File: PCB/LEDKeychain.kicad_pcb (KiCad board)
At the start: 2 copper layers, 32 x 49.5 mm, 37 parts, among them U1 13.56MHz

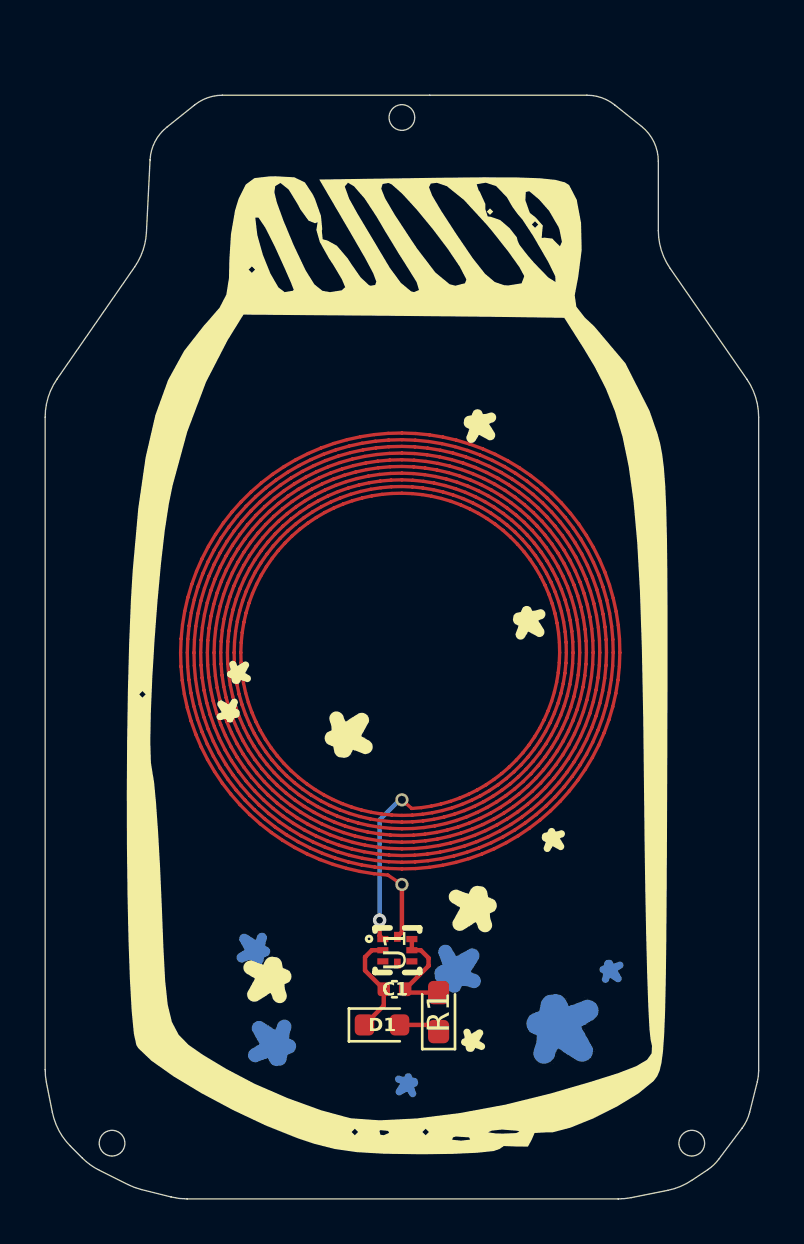
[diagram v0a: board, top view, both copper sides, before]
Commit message: Add files via upload
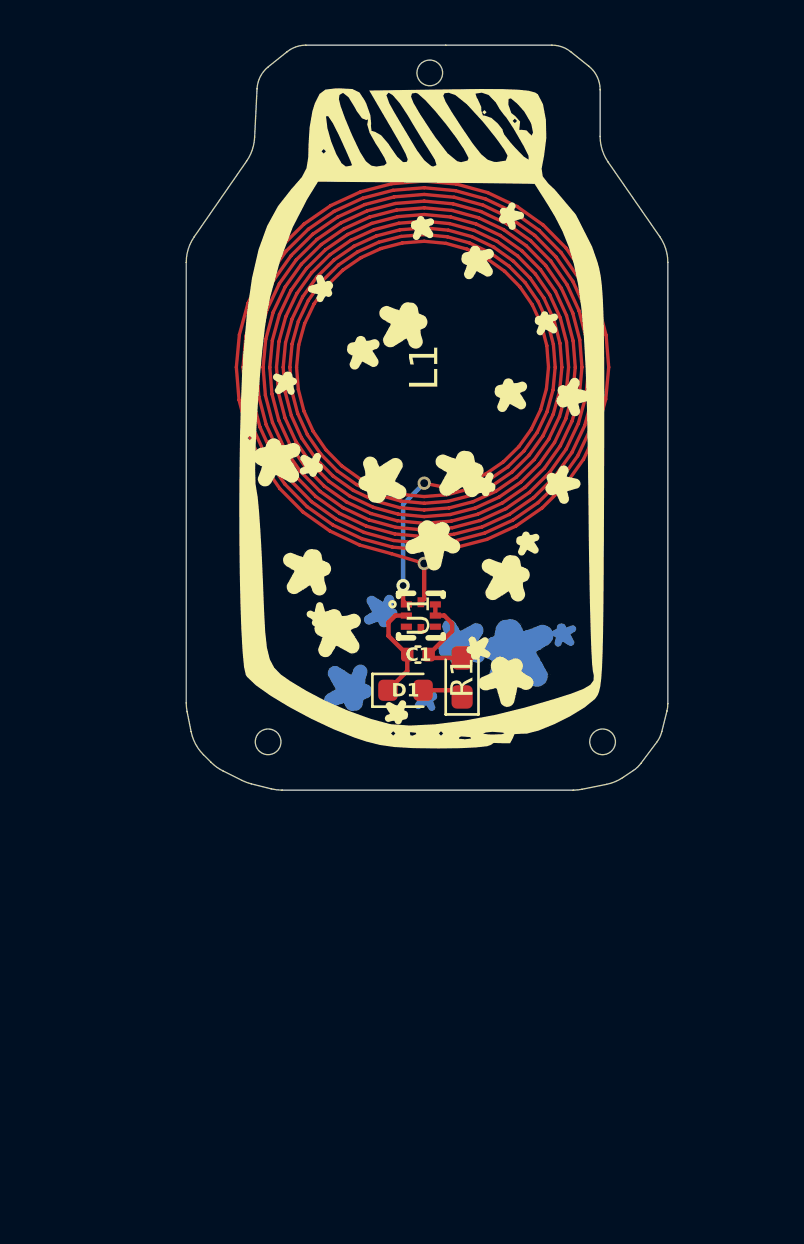
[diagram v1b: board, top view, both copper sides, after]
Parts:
- removed the REF** at (131.0, 93.0)
- removed the REF** at (144.0, 115.0)
- removed the REF** at (118.0, 115.0)
- removed the REF** at (131.0, 69.0)
- added G***: LOGO, LOGO, F.Cu at (137.7, 78.8)
- added G***: LOGO, LOGO, F.Cu at (125.8, 85.7)
- added G***: LOGO, LOGO, F.Cu at (134.5, 84.9)
- added G***: LOGO, LOGO, F.Cu at (130.5, 95.1)
- added G***: LOGO, LOGO, F.Cu at (136.4, 73.7)
- added G***: LOGO, LOGO, F.Cu at (128.5, 93.3)
- added G***: LOGO, LOGO, F.Cu at (129.6, 80.4)
- added G***: LOGO, LOGO, F.Cu at (127.6, 90.8)
- added G***: LOGO, LOGO, F.Cu at (139.5, 81.9)
- added G***: LOGO, LOGO, F.Cu at (129.9, 78.7)
- added G***: LOGO, LOGO, F.Cu at (139.0, 85.8)
- added G***: LOGO, LOGO, B.Cu at (133.7, 88.5)
- added G***: LOGO, LOGO, B.Cu at (135.7, 83.3)
- added G***: LOGO, LOGO, B.Cu at (130.0, 87.9)
- added G***: LOGO, LOGO, B.Cu at (136.8, 88.5)
- added G***: LOGO, LOGO, B.Cu at (128.0, 89.8)
- added G***: LOGO, LOGO, F.Cu at (132.4, 85.4)
- added G***: LOGO, LOGO, B.Cu at (131.9, 74.6)
- added G***: LOGO, LOGO, B.Cu at (126.4, 77.1)
- added G***: LOGO, LOGO, B.Cu at (127.7, 85.9)
- added G***: LOGO, LOGO, B.Cu at (132.3, 79.2)
- added G***: LOGO, LOGO, B.Cu at (138.4, 85.8)
- added G***: LOGO, LOGO, F.Cu at (135.1, 95.4)
- added G***: LOGO, LOGO, B.Cu at (137.2, 86.7)
- added G***: LOGO, LOGO, B.Cu at (136.3, 73.6)
- added G***: LOGO, LOGO, B.Cu at (125.2, 82.0)
- added G***: LOGO, LOGO, F.Cu at (132.1, 74.6)
- added G***: LOGO, LOGO, B.Cu at (135.1, 91.4)
- added G***: LOGO, LOGO, B.Cu at (129.5, 88.9)
- added G***: LOGO, LOGO, F.Cu at (131.8, 89.3)
- added G***: LOGO, LOGO, F.Cu at (125.2, 81.1)
- added G***: LOGO, LOGO, F.Cu at (126.8, 76.4)
- added L1: L, Antenna:Antenna_8500000x5500000mm, F.Cu at (132.0, 80.2)
- added REF**: ToolingHole_1.152mm, MountingHole:ToolingHole_1.152mm, F.Cu at (140.0, 97.0)
- added REF**: ToolingHole_1.152mm, MountingHole:ToolingHole_1.152mm, F.Cu at (125.0, 97.0)
- added REF**: ToolingHole_1.152mm, MountingHole:ToolingHole_1.152mm, F.Cu at (132.2, 67.0)
- G***: moved to B.Cu
- R1: value 51 -> 47
- moved G*** 19.3 mm to (125.8, 82.2)
- moved G*** 18.4 mm to (125.5, 89.8)
- moved G*** 17.6 mm to (135.0, 92.6)
- moved G*** 17.3 mm to (131.9, 95.7)
- moved G*** 16.9 mm to (138.0, 93.7) (x2)
- moved G*** 16.8 mm to (134.8, 94.7)
- moved G*** 16.3 mm to (127.4, 94.2) (x2)
- moved G*** 16.2 mm to (129.2, 90.8)
- moved G*** 15.9 mm to (129.1, 93.8)
- moved G*** 15.7 mm to (127.8, 93.0)
- moved G*** 15.2 mm to (138.9, 92.4)
- moved C1 15.0 mm to (131.7, 93.1)
- moved D1 15.0 mm to (131.2, 94.7)
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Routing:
- net Net-(U1-LA): track 6.78 -> 5.89 mm
- net Net-(U1-LB): track 2.43 -> 1.80 mm
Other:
- board size 32 x 49.5 mm -> 21.6 x 33.4 mm
